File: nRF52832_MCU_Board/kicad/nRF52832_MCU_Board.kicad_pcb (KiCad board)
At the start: 2 copper layers, 65 x 40 mm, 60 parts, among them J1 CONN_01X03, J2 CONN_01X16, J3 CONN_01X08, J4 CONN_01X03, J5 MICROUSB, J6 DEBUG_CONNECTOR, J7 CONN_01X05, J8 MM8130-2600, J9 CONN_01X08, U2 TLV1117, X1 32MHz, X2 32.768kHz

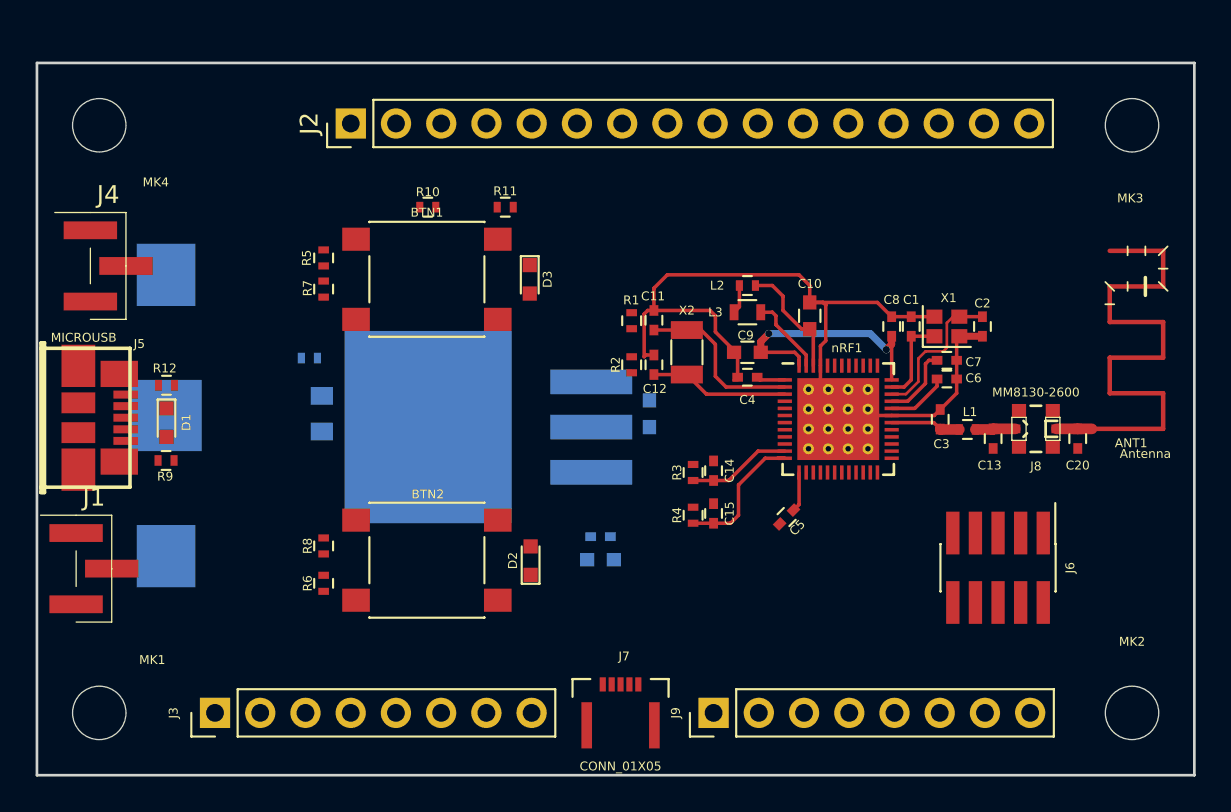
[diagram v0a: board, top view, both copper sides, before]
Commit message: Update KiCad project nRF52832_MCU_Board
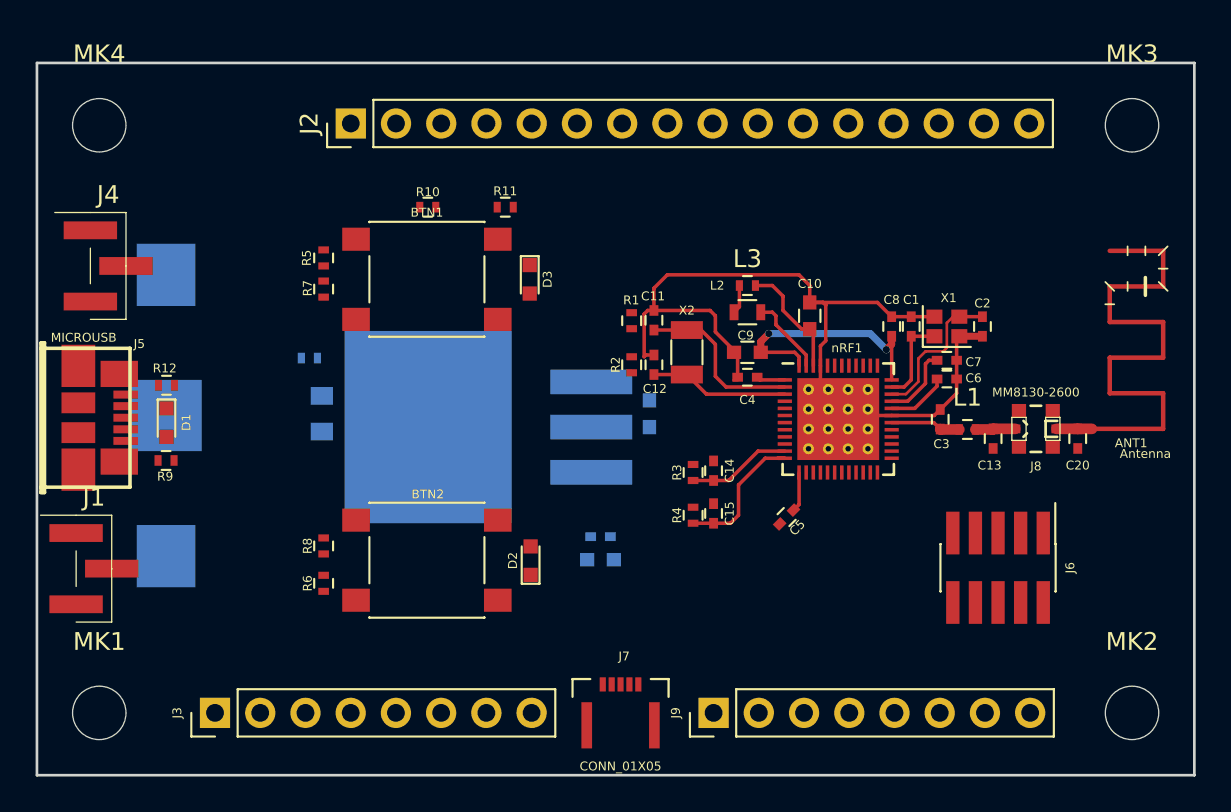
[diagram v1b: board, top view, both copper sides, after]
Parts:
- J2: footprint Pin_Headers:Pin_Header_Straight_1x16_Pitch2.54mm -> Nordic_misc:Pin_Header_Straight_1x16_Pitch2.54mm
- J3, J9: footprint Pin_Headers:Pin_Header_Straight_1x08_Pitch2.54mm -> Nordic_misc:Pin_Header_Straight_1x08_Pitch2.54mm
